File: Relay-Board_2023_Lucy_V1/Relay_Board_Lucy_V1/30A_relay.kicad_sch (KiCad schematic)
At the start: 5 parts, among them K5 J115F11CH12VDCS61.5, Q1 SI2302A-TPMSCT-ND

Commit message: updated, created gerbers, created p&p, created BOM's
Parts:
- D5: Part# digikey -> 478-7800-1-ND
- K5: Part# digikey -> 2449-J115F11CH12VDCS61.5-ND
- Q1: Part# digikey -> SI2302A-TPMSCT-ND
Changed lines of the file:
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@@
       (effects (font (size 1.27 1.27)) hide)
     )
-    (property "Part#" "digikey" (at 139.7 96.52 0)
+    (property "Part#" "2449-J115F11CH12VDCS61.5-ND" (at 139.7 96.52 0)
       (effects (font (size 1.27 1.27)) hide)
     )
@@
       (effects (font (size 1.27 1.27)) hide)
     )
-    (property "Part#" "digikey" (at 111.76 111.76 0)
+    (property "Part#" "SI2302A-TPMSCT-ND" (at 111.76 111.76 0)
       (effects (font (size 1.27 1.27)) hide)
     )
@@
       (effects (font (size 1.27 1.27)) hide)
     )
-    (property "Part#" "digikey" (at 114.3 96.52 0)
+    (property "Part#" "478-7800-1-ND" (at 114.3 96.52 0)
       (effects (font (size 1.27 1.27)) hide)
     )

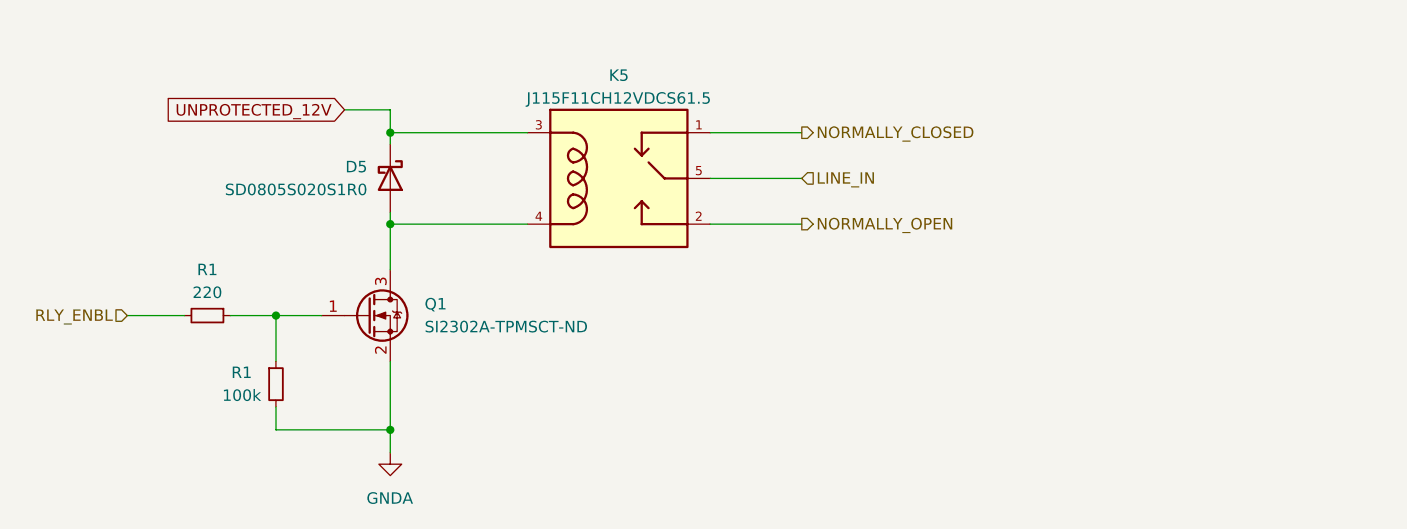
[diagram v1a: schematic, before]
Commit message: update
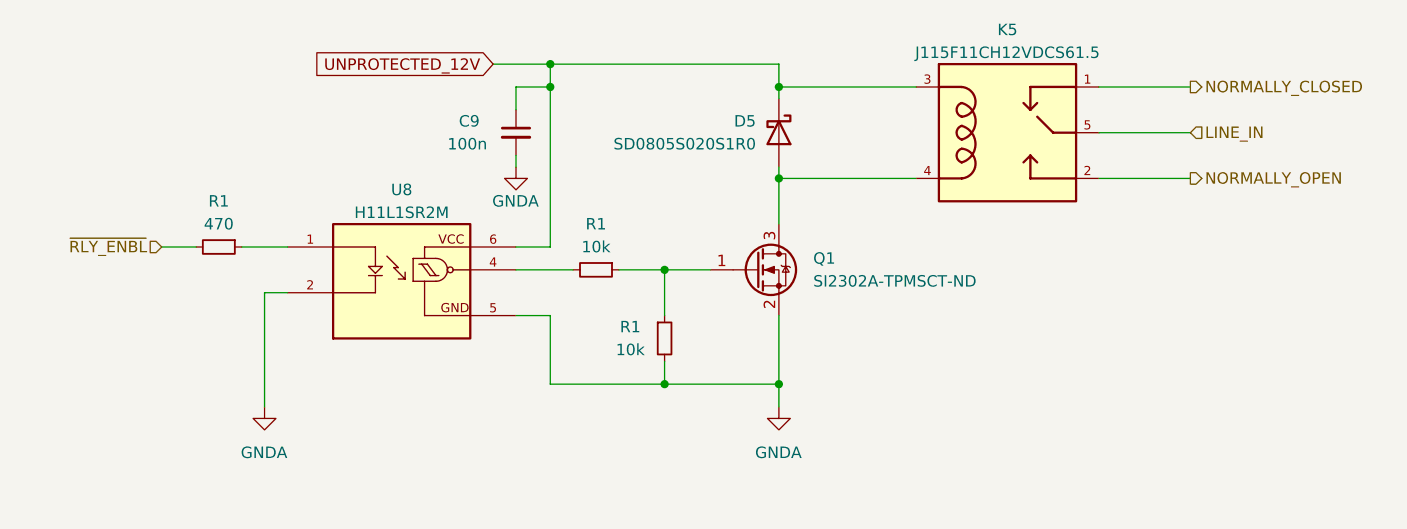
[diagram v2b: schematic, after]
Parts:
- added C9: 100n, Capacitor_SMD:C_0603_1608Metric, symbol Device:C_Small
- added R1: 470, Resistor_SMD:R_0603_1608Metric, symbol Device:R_Small
- added U8: H11L1SR2M, RB_FTP:IC_H11L1SR2M, symbol RB_PARTS:H11L1SR2M
- R1: value 220 -> 10k
- R1: value 100k -> 10k
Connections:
- net GNDA: now also C9.2, U8.2, U8.5
- net UNPROTECTED_12V: now also C9.1, U8.6
- net RLY_ENBL: no longer names the net of R1.2
- net RLY_ENBL: now also U8.4
- new net: R1.1, U8.1
- new net ~{RLY_ENBL}: R1.2
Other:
- moved on the sheet: D5, K5, Q1, R1
